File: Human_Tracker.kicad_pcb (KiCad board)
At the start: 4 copper layers, 200 x 50 mm, 59 parts, among them U1 TPS54233QDRQ1, U2 ICS-43434_C5656610, U3 ICS-43434_C5656610, U4 ADM7172ACPZ-3.3-R7, U5 BME680, U6 ESP32-S3-WROOM-1(N16R8), U7 MLX90640ESF-BAB-000-TU, U8 FRC0805F1400TS 140

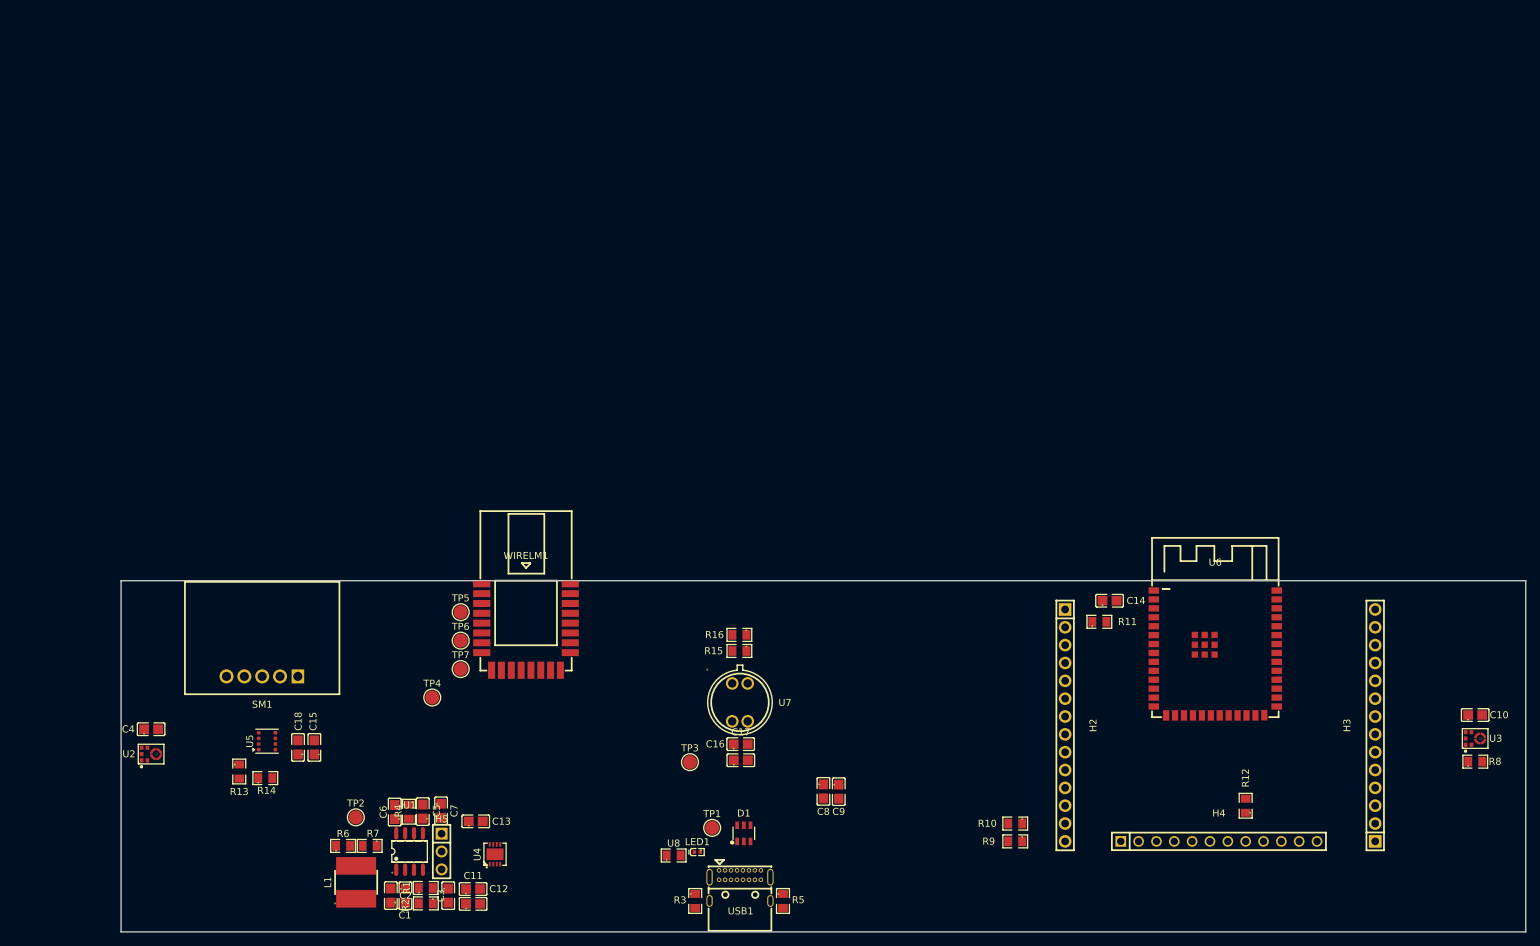
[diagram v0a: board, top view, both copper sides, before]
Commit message: caca
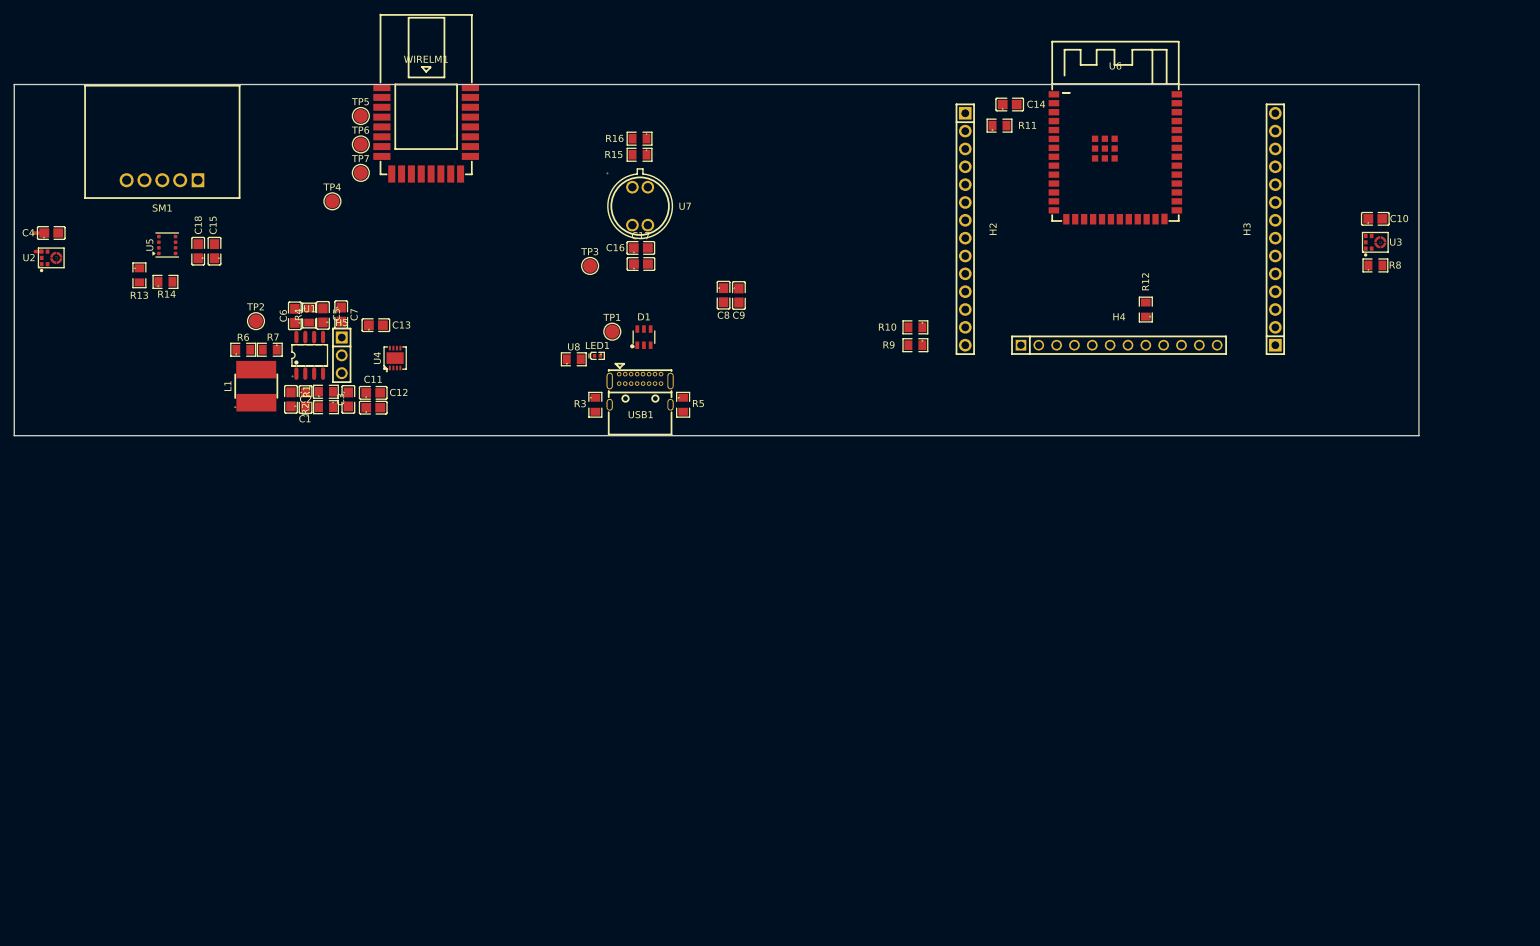
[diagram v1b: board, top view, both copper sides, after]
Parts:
- moved C13 72.1 mm to (101.5, 59.3)
- moved C5 72.1 mm to (94.0, 57.9)
- moved L1 72.1 mm to (84.5, 67.9)
- moved U1 72.1 mm to (92.1, 63.6)
- moved WIRELM1 72.1 mm to (108.7, 31.6)
- moved C1 72.1 mm to (91.5, 69.9)
- moved C11 72.1 mm to (101.1, 71.0)
- moved C12 72.1 mm to (101.1, 68.9)
- moved C14 72.1 mm to (191.7, 27.9)
- moved C15 72.1 mm to (78.5, 48.7)
- moved C16 72.1 mm to (139.2, 48.3)
- moved C18 72.1 mm to (76.2, 48.7)
- moved C2 72.1 mm to (89.4, 69.8)
- moved C3 72.1 mm to (97.6, 69.8)
- moved C7 72.1 mm to (96.6, 57.8)
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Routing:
- net +3.3V: track 0.00 -> 2.83 mm
- added copper zone on In2.Cu, net +3.3V
- added copper zone on In1.Cu, net GND
